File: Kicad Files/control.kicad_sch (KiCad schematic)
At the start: 77 parts, among them U42 74LS161, U43 SST39SF020, U44 SST39SF020, U45 SST39SF020, U46 SST39SF020

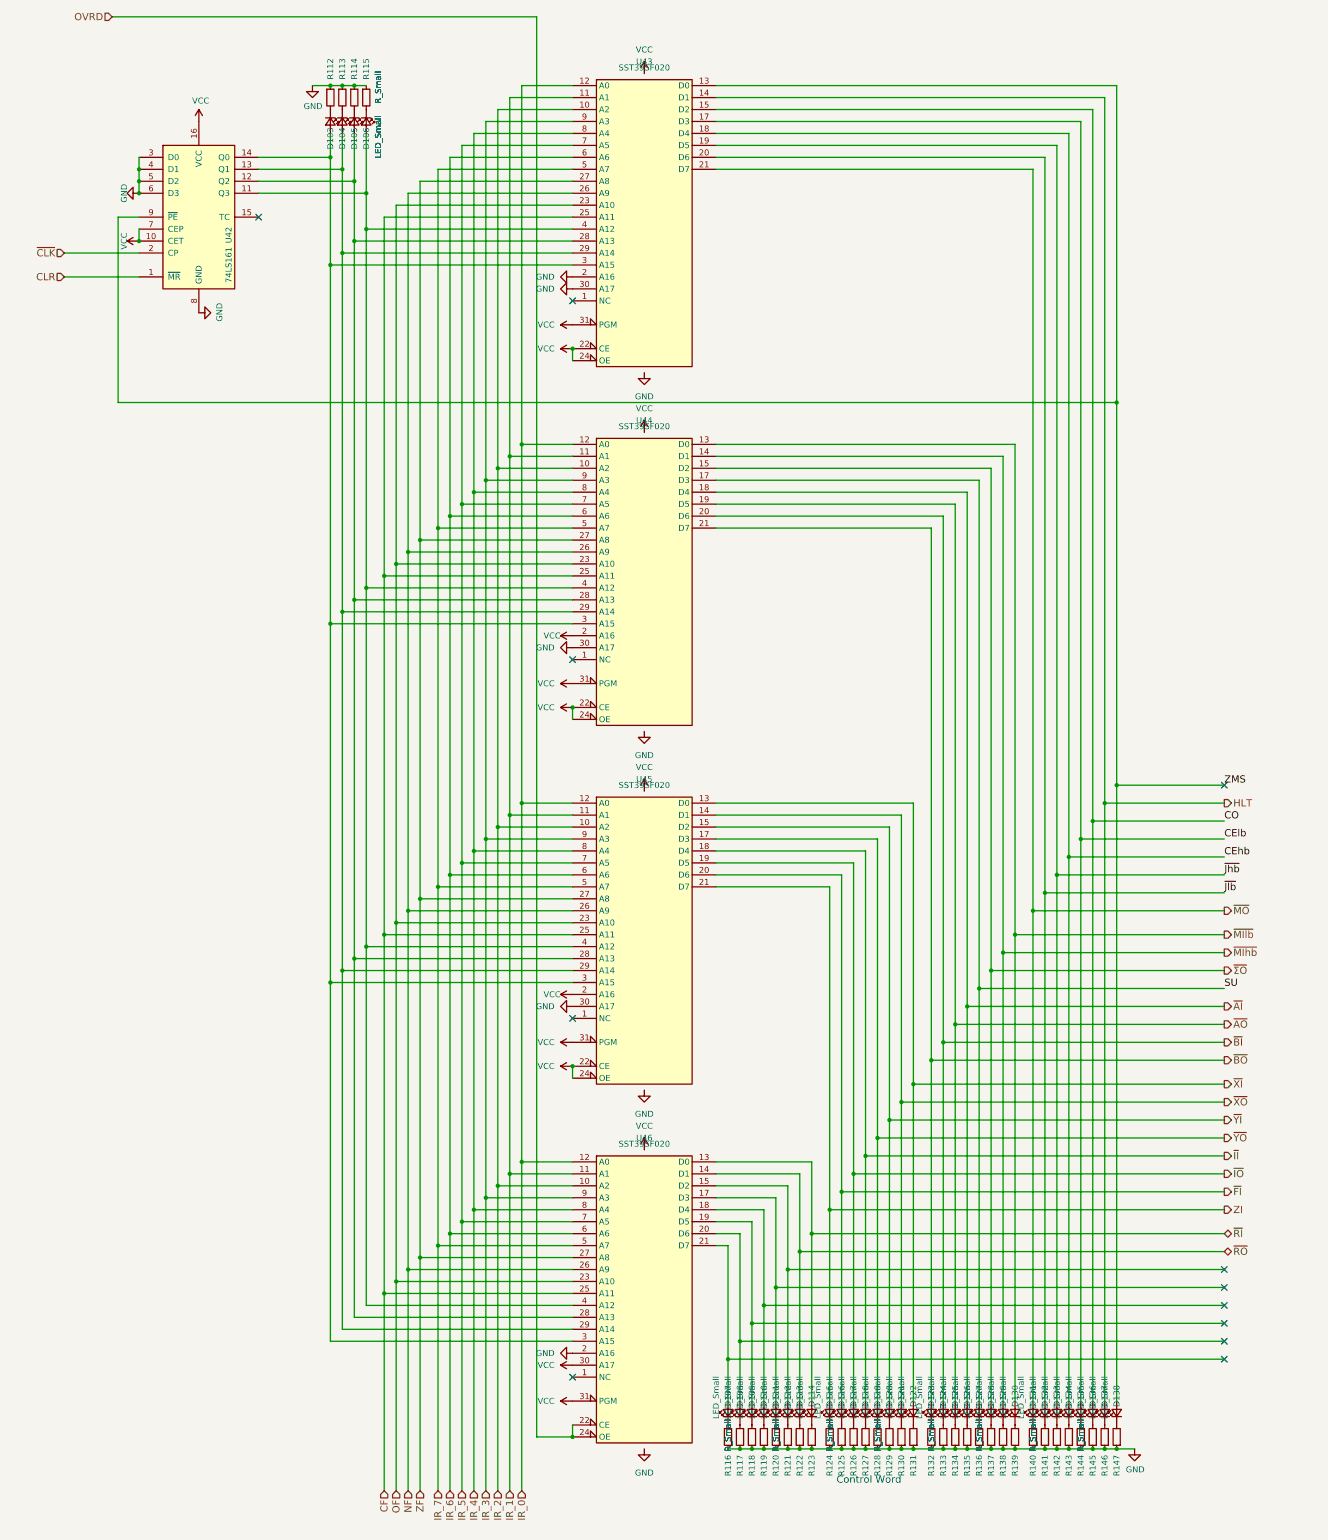
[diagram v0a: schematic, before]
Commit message: new control sigs
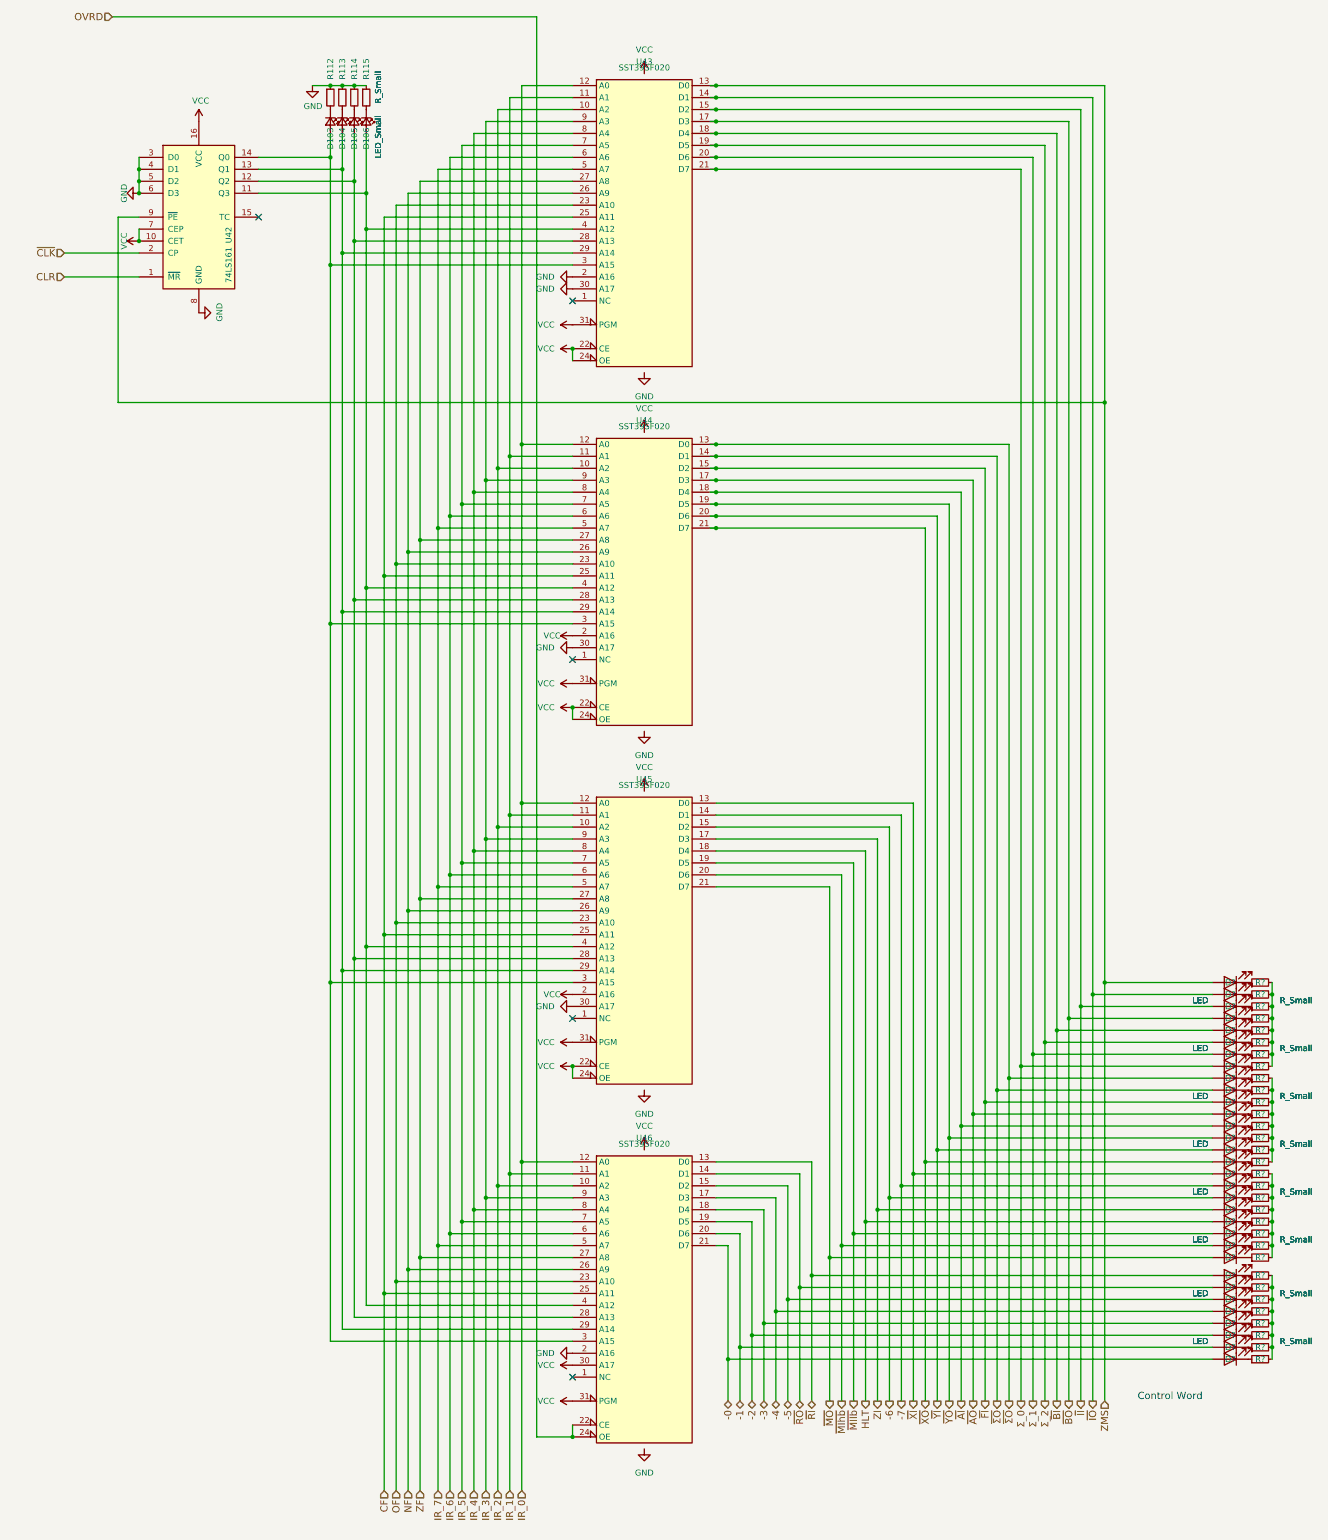
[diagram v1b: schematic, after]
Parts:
- removed D107, D108, D109, D110, D111, D112, D113, D114, D115, D116, D117, D118, D119, D120, D121, D122, D123, D124, D125, D126, D127, D128, D129, D130, D131, D132, D133, D134, D135, D136, D137, D138: LED_Small, symbol Device:LED_Small
- removed R116, R117, R118, R119, R120, R121, R122, R123, R124, R125, R126, R127, R128, R129, R130, R131, R132, R133, R134, R135, R136, R137, R138, R139, R140, R141, R142, R143, R144, R145, R146, R147: R_Small, symbol Device:R_Small
- added D? (x32): LED, symbol Device:LED
- added R? (x32): R_Small, symbol Device:R_Small
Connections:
- net CEhb is gone; now on net ~{BI}: U43.18 (D4)
- net CElb is gone; now on net ~{BO}: U43.17 (D3)
- net CO is gone; now on net ~{II}: U43.15 (D2)
- net SU is gone; now on net ~{AO}: U44.17 (D3)
- net HLT: now also U45.18 (D4), D?.2 (A); no longer U43.14 (D1)
- net ZI: now also U45.17 (D3), D?.2 (A); no longer U45.21 (D7)
- net ZMS: now also D?.2 (A)
- net ~{AI}: now also D?.2 (A)
- net ~{AO}: now also D?.2 (A); no longer U44.19 (D5)
- net ~{BI}: now also D?.2 (A); no longer U44.20 (D6)
- net ~{BO}: now also D?.2 (A); no longer U44.21 (D7)
- net ~{FI}: now also U44.15 (D2), D?.2 (A); no longer U45.20 (D6)
- net ~{II}: now also D?.2 (A); no longer U45.18 (D4)
- net ~{IO}: now also U43.14 (D1), D?.2 (A); no longer U45.19 (D5)
- net ~{MIhb}: now also U45.20 (D6), D?.2 (A); no longer U44.14 (D1)
- net ~{MIlb}: now also U45.19 (D5), D?.2 (A); no longer U44.13 (D0)
- net ~{MO}: now also U45.21 (D7), D?.2 (A); no longer U43.21 (D7)
- net ~{RI}: now also D?.2 (A)
- net ~{RO}: now also D?.2 (A)
- net ~{XI}: now also D?.2 (A)
- net ~{XO}: now also U44.21 (D7), D?.2 (A); no longer U45.14 (D1)
- net ~{YI}: now also U44.20 (D6), D?.2 (A); no longer U45.15 (D2)
- net ~{YO}: now also U44.19 (D5), D?.2 (A); no longer U45.17 (D3)
- net ~{ΣO}: now also U44.13 (D0), U44.14 (D1), D?.2 (A), D?.2 (A); no longer U44.15 (D2)
- net -1: now reaches U46.20 (D6)
- net -1: now also D?.2 (A)
- net -2: now reaches U46.19 (D5)
- net -2: now also D?.2 (A)
- net -3: now reaches U46.18 (D4)
- net -3: now also D?.2 (A)
- net -4: now reaches U46.17 (D3)
- net -4: now also D?.2 (A)
- net -5: now reaches U46.15 (D2)
- net -5: now also D?.2 (A)
- net -0: now reaches U46.21 (D7)
- net -0: now also D?.2 (A)
- net ~{Jhb} renamed Σ_2
- net Σ_2: now also D?.2 (A)
- net ~{Jlb} renamed Σ_1
- net Σ_1: now also D?.2 (A)
- new net: D?.1 (K), R?.1 (x32)
- new net: R?.2, R?.2, R?.2, R?.2, R?.2, R?.2, R?.2, R?.2 (x4)
- new net -6: D?.2 (A), U45.15 (D2)
- new net -7: D?.2 (A), U45.14 (D1)
- new net Σ_0: D?.2 (A), U43.21 (D7)
- no-connect marks 12 -> 5
